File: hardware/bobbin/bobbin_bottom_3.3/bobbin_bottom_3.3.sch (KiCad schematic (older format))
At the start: 2 parts

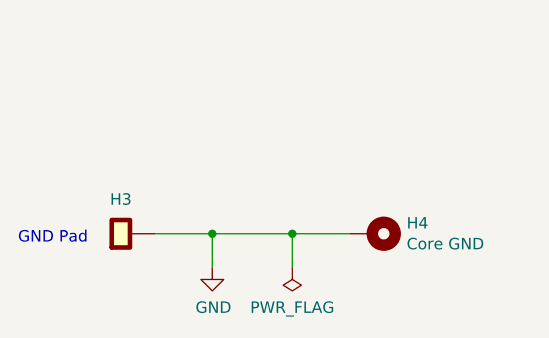
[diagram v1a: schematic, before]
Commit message: Bobbin bottom new scheme
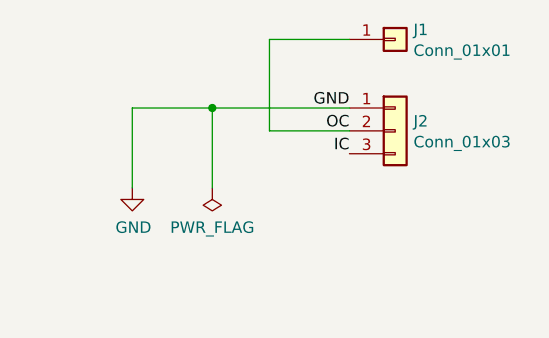
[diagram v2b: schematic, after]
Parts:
- removed H3: single_pad_smd, cycfi_library:round-single-pad-1.8mm-th, symbol cycfi_library:single_pad_smd
- removed H4: Core GND, cycfi_library:single-pad-10x2, symbol Mechanical:MountingHole_Pad
- added J1: Conn_01x01, cycfi_library:xr2-oc-coil-connector, symbol Connector_Generic:Conn_01x01
- added J2: Conn_01x03, cycfi_library:xr2-coil-connector, symbol Connector_Generic:Conn_01x03
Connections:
- net GND: now also J2.1 (Pin_1)
- new net IC: J2.3 (Pin_3)
- new net OC: J1.1 (Pin_1), J2.2 (Pin_2)
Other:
- note removed: "GND Pad"
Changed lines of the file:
@@
 $EndDescr
 $Comp
-L power:GND #PWR02
+L power:GND #PWR01
 U 1 1 60D88DF5
-P 5200 3350
-F 0 "#PWR02" H 5200 3100 50  0001 C CNN
-F 1 "GND" H 5205 3177 50  0000 C CNN
-F 2 "" H 5200 3350 50  0001 C CNN
-F 3 "" H 5200 3350 50  0001 C CNN
-	1    5200 3350
+P 4850 3000
+F 0 "#PWR01" H 4850 2750 50  0001 C CNN
+F 1 "GND" H 4855 2827 50  0000 C CNN
+F 2 "" H 4850 3000 50  0001 C CNN
+F 3 "" H 4850 3000 50  0001 C CNN
+	1    4850 3000
 	1    0    0    -1
 $EndComp
 $Comp
-L power:PWR_FLAG #FLG0101
+L power:PWR_FLAG #FLG01
 U 1 1 60D8CE57
-P 5550 3350
-F 0 "#FLG0101" H 5550 3425 50  0001 C CNN
-F 1 "PWR_FLAG" H 5550 3523 50  0000 C CNN
-F 2 "" H 5550 3350 50  0001 C CNN
-F 3 "~" H 5550 3350 50  0001 C CNN
-	1    5550 3350
+P 5200 3000
+F 0 "#FLG01" H 5200 3075 50  0001 C CNN
+F 1 "PWR_FLAG" H 5200 3173 50  0000 C CNN
+F 2 "" H 5200 3000 50  0001 C CNN
+F 3 "~" H 5200 3000 50  0001 C CNN
+	1    5200 3000
 	-1   0    0    1
 $EndComp
+$Comp
+L Connector_Generic:Conn_01x01 J1
+U 1 1 6150EC9C
+P 6000 2350
+F 0 "J1" H 6080 2392 50  0000 L CNN
+F 1 "Conn_01x01" H 6080 2301 50  0000 L CNN
+F 2 "cycfi_library:xr2-oc-coil-connector" H 6000 2350 50  0001 C CNN
+F 3 "~" H 6000 2350 50  0001 C CNN
+	1    6000 2350
+	1    0    0    -1
+$EndComp
 Wire Wire Line
-	5550 3200 5200 3200
+	4850 2650 5200 2650
+Wire Wire Line
+	4850 2650 4850 3000
+Wire Wire Line
+	5200 2650 5200 3000
 $Comp
-L cycfi_library:single_pad_smd H3
-U 1 1 60D997A7
-P 4850 3200
-F 0 "H3" V 5000 3250 50  0000 C CNN
-F 1 "single_pad_smd" H 4850 3400 50  0001 C CNN
-F 2 "cycfi_library:round-single-pad-1.8mm-th" H 4850 3200 50  0001 C CNN
-F 3 "~" H 4850 3200 50  0001 C CNN
-	1    4850 3200
-	0    -1   -1   0
+L Connector_Generic:Conn_01x03 J2
+U 1 1 615174B9
+P 6000 2750
+F 0 "J2" H 6080 2792 50  0000 L CNN
+F 1 "Conn_01x03" H 6080 2701 50  0000 L CNN
+F 2 "cycfi_library:xr2-coil-connector" H 6000 2750 50  0001 C CNN
+F 3 "~" H 6000 2750 50  0001 C CNN
+	1    6000 2750
+	1    0    0    -1
 $EndComp
-Connection ~ 5200 3200
+Connection ~ 5200 2650
 Wire Wire Line
-	5200 3350 5200 3200
+	5200 2650 5800 2650
 Wire Wire Line
-	5550 3350 5550 3200
-Text Notes 4350 3250 0    50   ~ 0
-GND Pad
+	5800 2750 5450 2750
 Wire Wire Line
-	4950 3200 5200 3200
-Connection ~ 5550 3200
+	5450 2750 5450 2350
 Wire Wire Line
-	5800 3200 5550 3200
-$Comp
-L Mechanical:MountingHole_Pad H4
-U 1 1 60D8FEDB
-P 5900 3200
-F 0 "H4" V 5854 3350 50  0000 L CNN
-F 1 "Core GND" V 5945 3350 50  0000 L CNN
-F 2 "cycfi_library:single-pad-10x2" H 5900 3200 50  0001 C CNN
-F 3 "~" H 5900 3200 50  0001 C CNN
-	1    5900 3200
-	0    1    1    0
-$EndComp
+	5450 2350 5800 2350
+Text Label 5800 2650 2    50   ~ 0
+GND
+Text Label 5800 2750 2    50   ~ 0
+OC
+Text Label 5800 2850 2    50   ~ 0
+IC
 $EndSCHEMATC
